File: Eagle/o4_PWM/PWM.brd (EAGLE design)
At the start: 160 x 100 mm, 10 parts, among them IC1 TINY13-20SSU

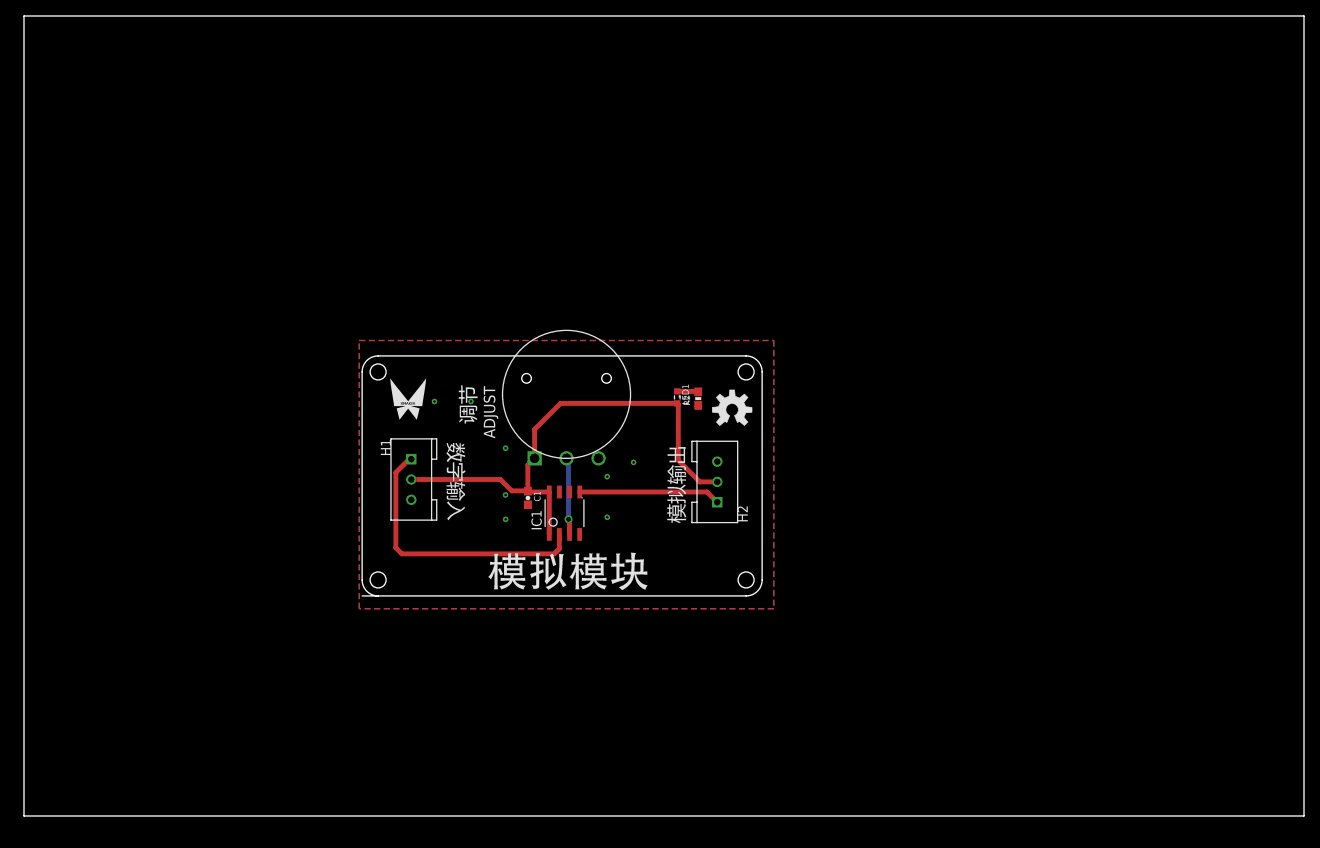
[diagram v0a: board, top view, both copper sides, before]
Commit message: 第一次更新
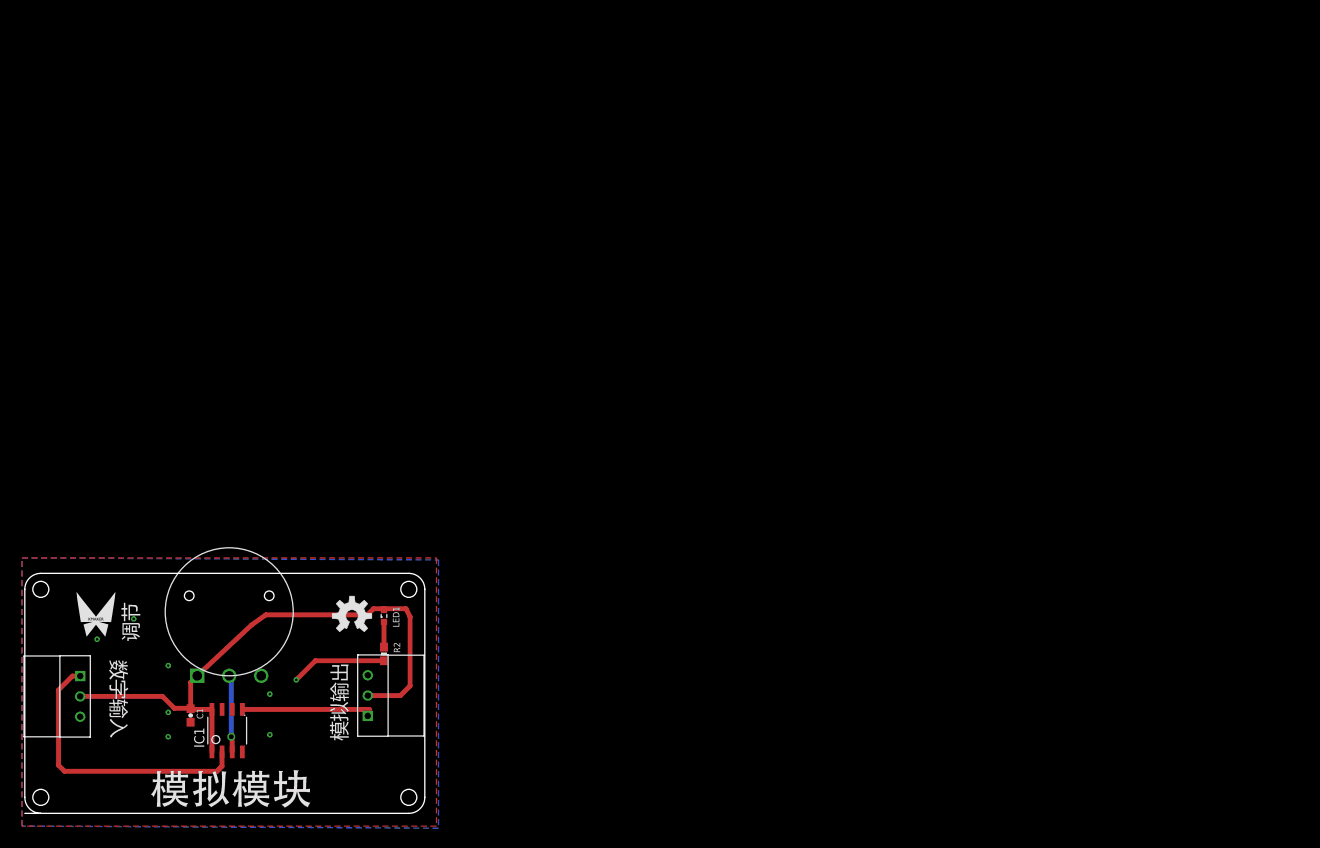
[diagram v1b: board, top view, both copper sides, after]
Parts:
- removed H1, H2: HEAD_LOCK, HEAD_LOCK:HEAD_LOCK
- added HEAD_LOCK1, HEAD_LOCK2: HEAD_LOCK, Xmaker_yuhui:HEAD_LOCK
- U$2: value XMAKERLOGO2 -> XMAKERLOGO_5MM_TOP; device Xmaker_yuhui:XMAKERLOGO2 -> Xmaker_yuhui:XMAKERLOGO_5MM_TOP
- U$4: value OPENHARDWARE -> OPENHARDWARE_5MM_TOP; device Xmaker_yuhui:OPENHARDWARE -> Xmaker_yuhui:OPENSOURCE_5MM_TOP
- moved U$4 54.1 mm to (41.0, 25.0)
- moved R2 50.6 mm to (45.0, 20.3)
- moved U$1 50.2 mm to (25.7, 17.5)
- moved C1 50.2 mm to (20.8, 12.6)
- moved IC1 50.2 mm to (25.4, 10.7)
- moved U$3 50.2 mm to (0.10, 0.33)
- moved LED1 45.7 mm to (45.0, 25.0), turned to 90 degrees
- moved U$2 42.6 mm to (9.00, 25.0)
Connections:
- net ADC: now also HEAD_LOCK1.1; no longer H1.1
- net GND: now also HEAD_LOCK1.3, HEAD_LOCK2.3; no longer H1.3, H2.3
- net PWM: now also HEAD_LOCK2.1; no longer H2.1
- net VCC: now also HEAD_LOCK1.2, HEAD_LOCK2.2; no longer H1.2, H2.2
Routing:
- net GND: track 0.00 -> 12.0 mm
- net VCC: track 63.6 -> 71.9 mm
- net ADC: track 36.2 -> 37.0 mm
- net PWM: track 17.7 -> 17.0 mm
- net N$1: track 2.64 -> 3.15 mm
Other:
- board size 160 x 100 mm -> 50 x 30 mm
- board text removed: "ADJUST"
- board text removed: "INPUT"
- board text removed: "OUTPUT"

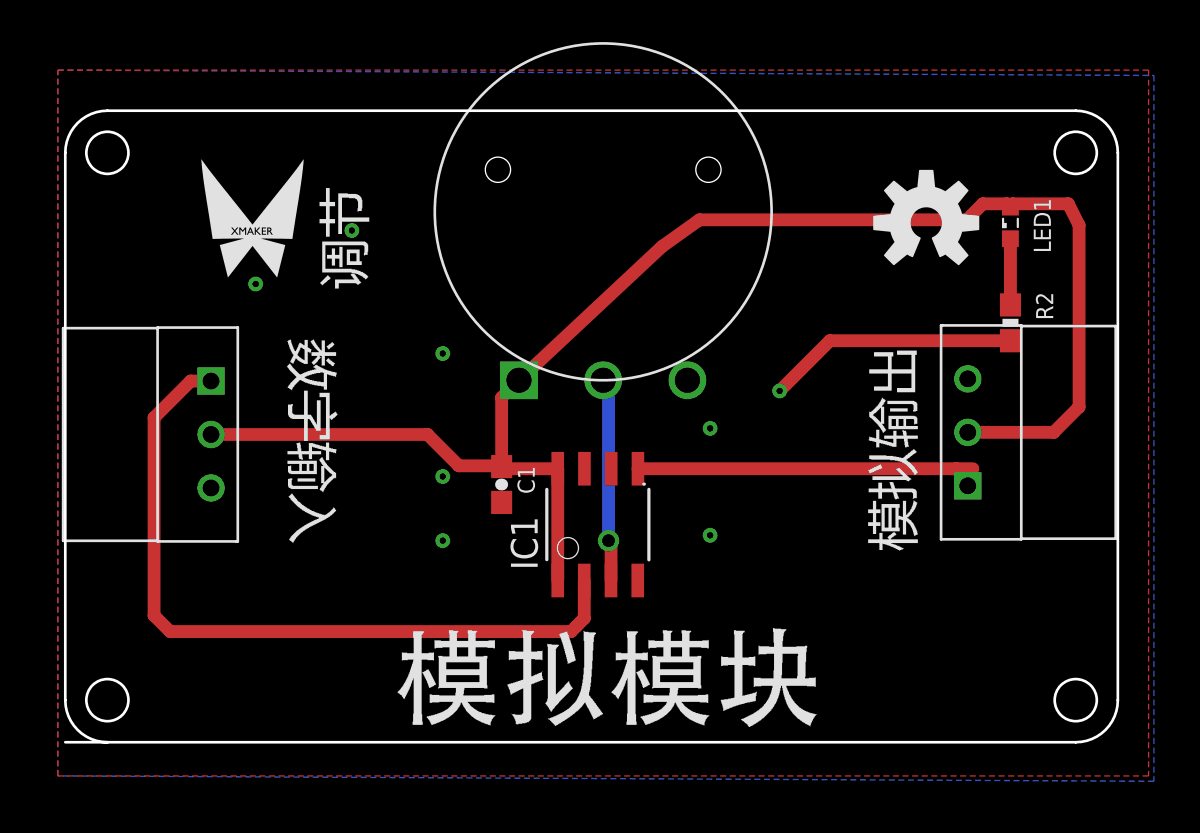
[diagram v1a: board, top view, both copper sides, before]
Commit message: 12.15
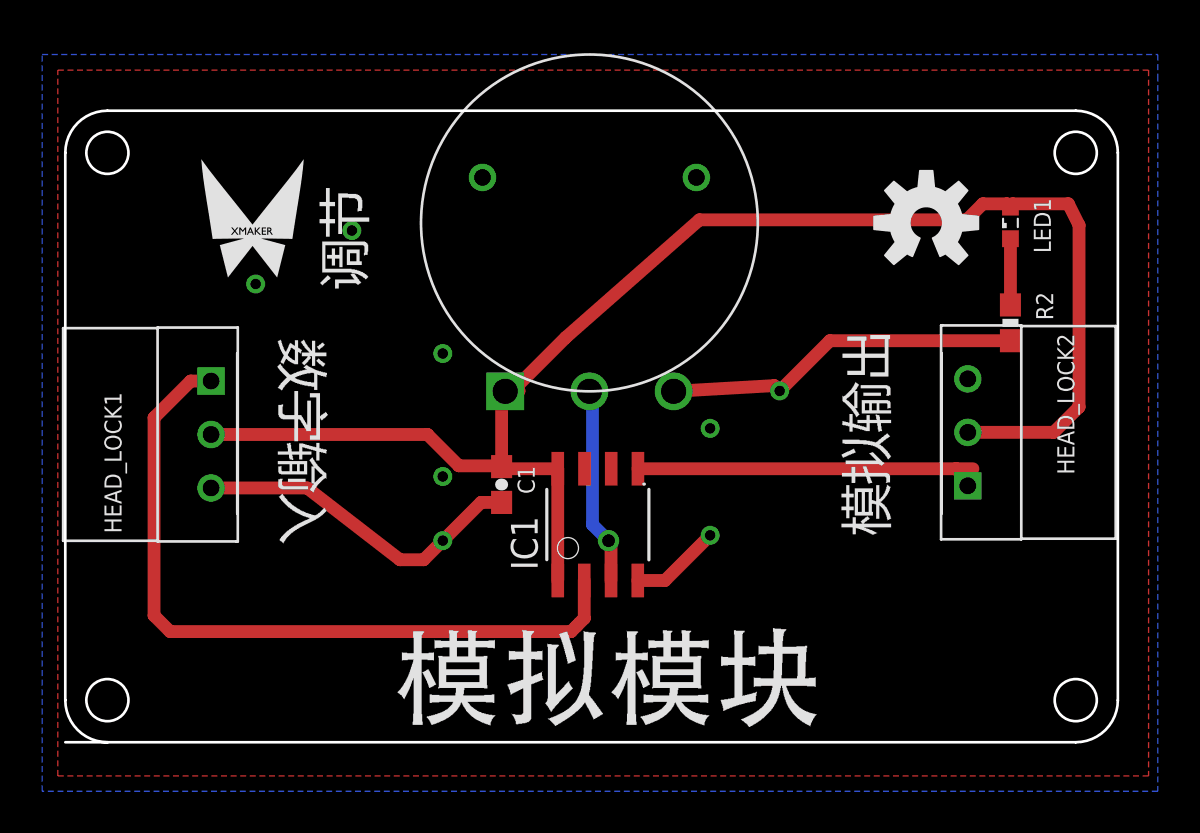
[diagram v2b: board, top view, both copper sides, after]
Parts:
- removed U$1: POL_CIRCLE, Xmaker_yuhui:POT_CIRCLE
- added U$5: POL_CIRCLE, Xmaker:POT_CIRCLE
- HEAD_LOCK1, HEAD_LOCK2: device Xmaker_yuhui:HEAD_LOCK -> Xmaker:HEAD_LOCK
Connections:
- net CONTROL: now also U$5.P$2; no longer U$1.P$2
- net GND: now also U$5.P$3; no longer U$1.P$3
- net VCC: now also U$5.P$1; no longer U$1.P$1
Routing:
- net GND: track 12.0 -> 37.5 mm
- net VCC: track 71.9 -> 73.0 mm
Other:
- board text removed: "GND"
- board text removed: "SIG"
- board text removed: "VCC"
